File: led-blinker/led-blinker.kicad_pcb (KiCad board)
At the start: 2 copper layers, 3 parts, among them J1 Conn_01x02_Male

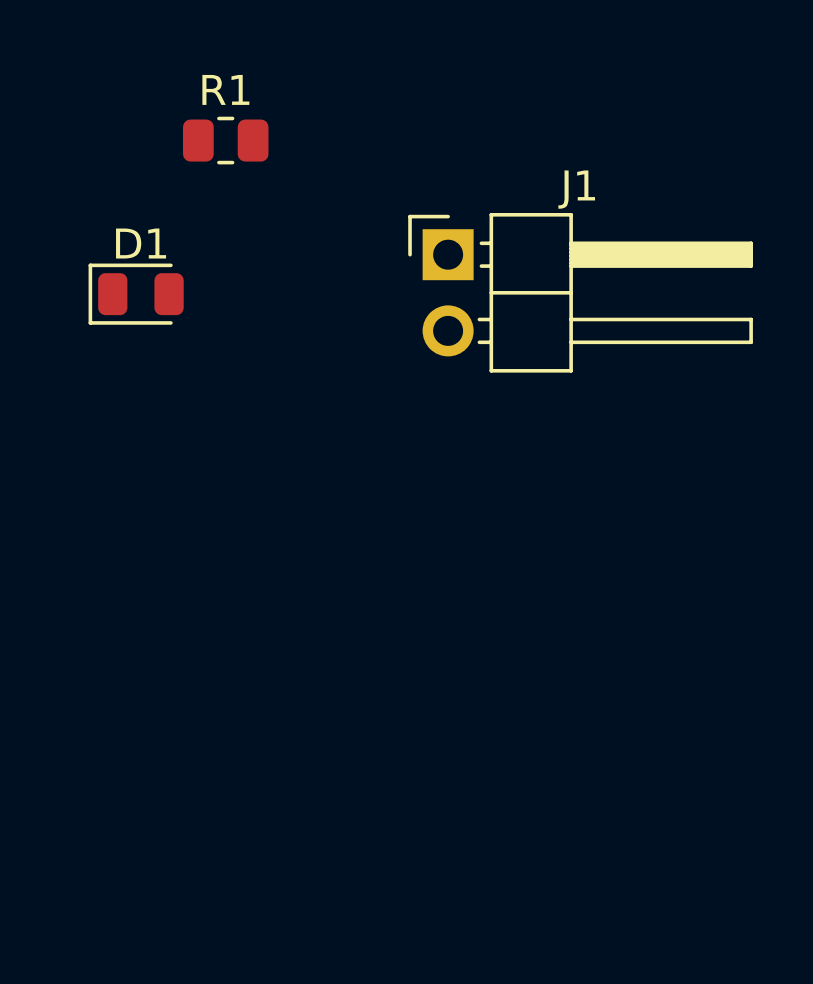
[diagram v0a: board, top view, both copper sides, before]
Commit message: Update led-blinker.kicad_pcb
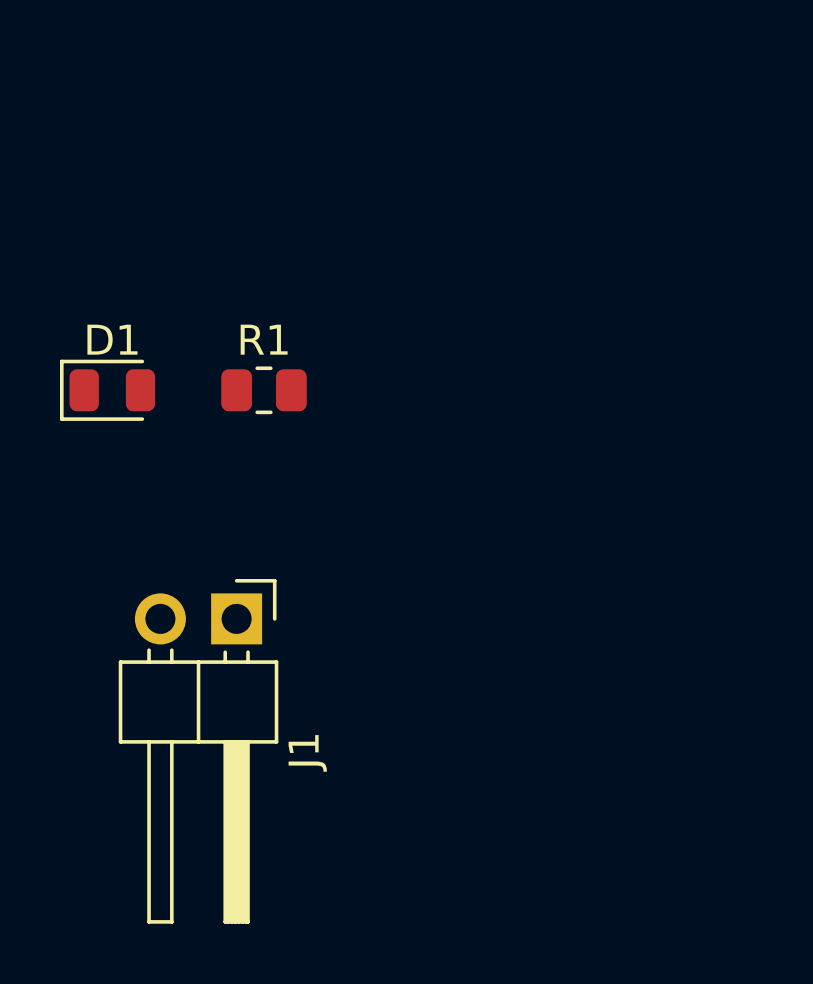
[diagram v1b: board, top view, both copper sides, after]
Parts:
- moved J1 14.0 mm to (125.7, 115.0), turned to -90 degrees
- moved R1 8.42 mm to (126.6, 107.4)
- moved D1 3.34 mm to (121.6, 107.4)
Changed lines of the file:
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@@
   (net 3 "Net-(J1-Pad1)")
   (footprint "LED_SMD:LED_0805_2012Metric" (layer "F.Cu")
-    (at 122.545 104.18)
+    (at 121.5925 107.385)
     (descr "LED SMD 0805 (2012 Metric), square (rectangular) end terminal, IPC_7351 nominal, (Body size source: https://docs.google.com/spreadsheets/d/1BsfQQcO9C6DZCsRaXUlFlo91Tg2WpOkGARC1WS5S8t0/edit?usp=sharing), generated with kicad-footprint-generator")
     (tags "LED")
@@
   )
   (footprint "Resistor_SMD:R_0805_2012Metric" (layer "F.Cu")
-    (at 125.3725 99.06)
+    (at 126.6475 107.385)
     (descr "Resistor SMD 0805 (2012 Metric), square (rectangular) end terminal, IPC_7351 nominal, (Body size source: IPC-SM-782 page 72, https://www.pcb-3d.com/wordpress/wp-content/uploads/ipc-sm-782a_amendment_1_and_2.pdf), generated with kicad-footprint-generator")
     (tags "resistor")
@@
   )
   (footprint "Connector_PinHeader_2.54mm:PinHeader_1x02_P2.54mm_Horizontal" (layer "F.Cu")
-    (at 132.785 102.865)
+    (at 125.735 115.005 -90)
     (descr "Through hole angled pin header, 1x02, 2.54mm pitch, 6mm pin length, single row")
     (tags "Through hole angled pin header THT 1x02 2.54mm single row")
@@
     (property "Sheetname" "")
     (attr through_hole)
-    (fp_text reference "J1" (at 4.385 -2.27) (layer "F.SilkS")
+    (fp_text reference "J1" (at 4.385 -2.27 90) (layer "F.SilkS")
       (effects (font (size 1 1) (thickness 0.15)))
     )
-    (fp_text value "Conn_01x02_Male" (at 4.385 4.81) (layer "F.Fab")
+    (fp_text value "Conn_01x02_Male" (at 4.385 4.81 90) (layer "F.Fab")
       (effects (font (size 1 1) (thickness 0.15)))
     )
-    (fp_text user "${REFERENCE}" (at 2.77 1.27 90) (layer "F.Fab")
+    (fp_text user "${REFERENCE}" (at 2.77 1.27) (layer "F.Fab")
       (effects (font (size 1 1) (thickness 0.15)))
     )
@@
     (fp_line (start -0.32 -0.32) (end -0.32 0.32) (layer "F.Fab") (width 0.1))
     (fp_line (start 1.5 3.81) (end 1.5 -0.635) (layer "F.Fab") (width 0.1))
-    (pad "1" thru_hole rect (at 0 0) (size 1.7 1.7) (drill 1) (layers *.Cu *.Mask)
+    (pad "1" thru_hole rect (at 0 0 270) (size 1.7 1.7) (drill 1) (layers *.Cu *.Mask)
       (net 3 "Net-(J1-Pad1)") (pinfunction "Pin_1") (pintype "passive"))
-    (pad "2" thru_hole oval (at 0 2.54) (size 1.7 1.7) (drill 1) (layers *.Cu *.Mask)
+    (pad "2" thru_hole oval (at 0 2.54 270) (size 1.7 1.7) (drill 1) (layers *.Cu *.Mask)
       (net 1 "Net-(J1-Pad2)") (pinfunction "Pin_2") (pintype "passive"))
     (model "${KICAD6_3DMODEL_DIR}/Connector_PinHeader_2.54mm.3dshapes/PinHeader_1x02_P2.54mm_Horizontal.wrl"
